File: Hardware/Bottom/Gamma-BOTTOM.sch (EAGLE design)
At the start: 33 parts

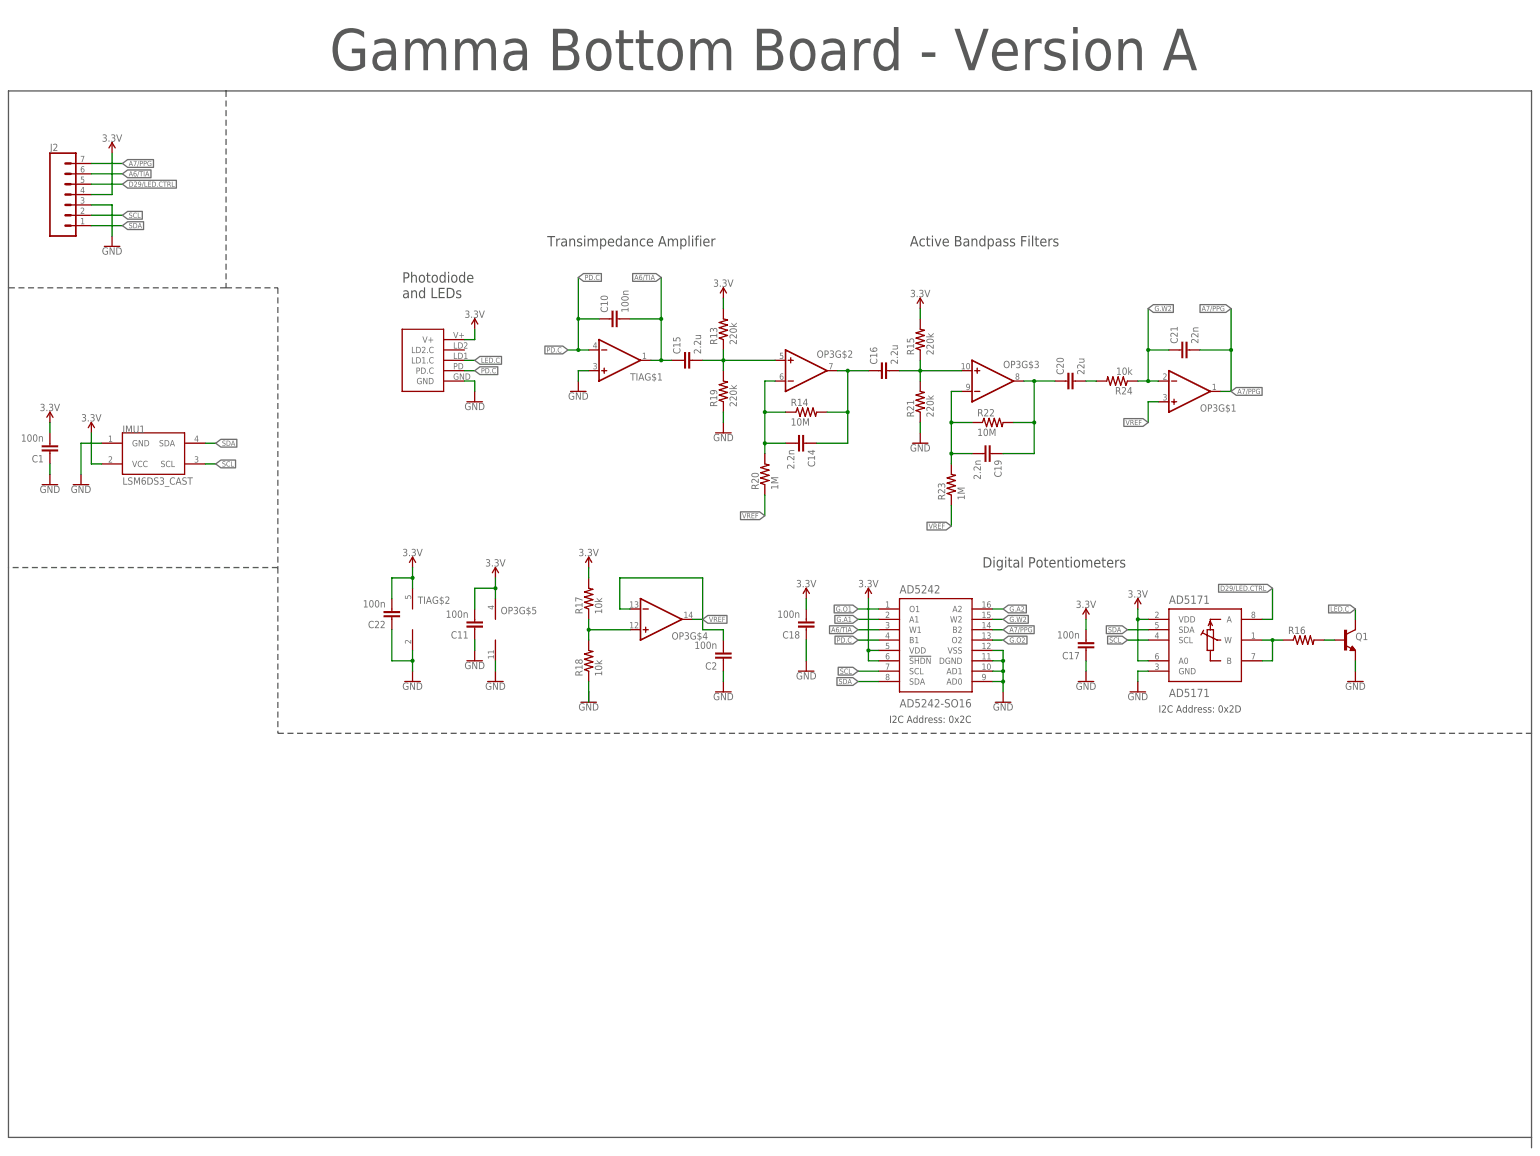
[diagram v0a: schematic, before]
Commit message: Pushed Changes to where I'm at (Take 007)
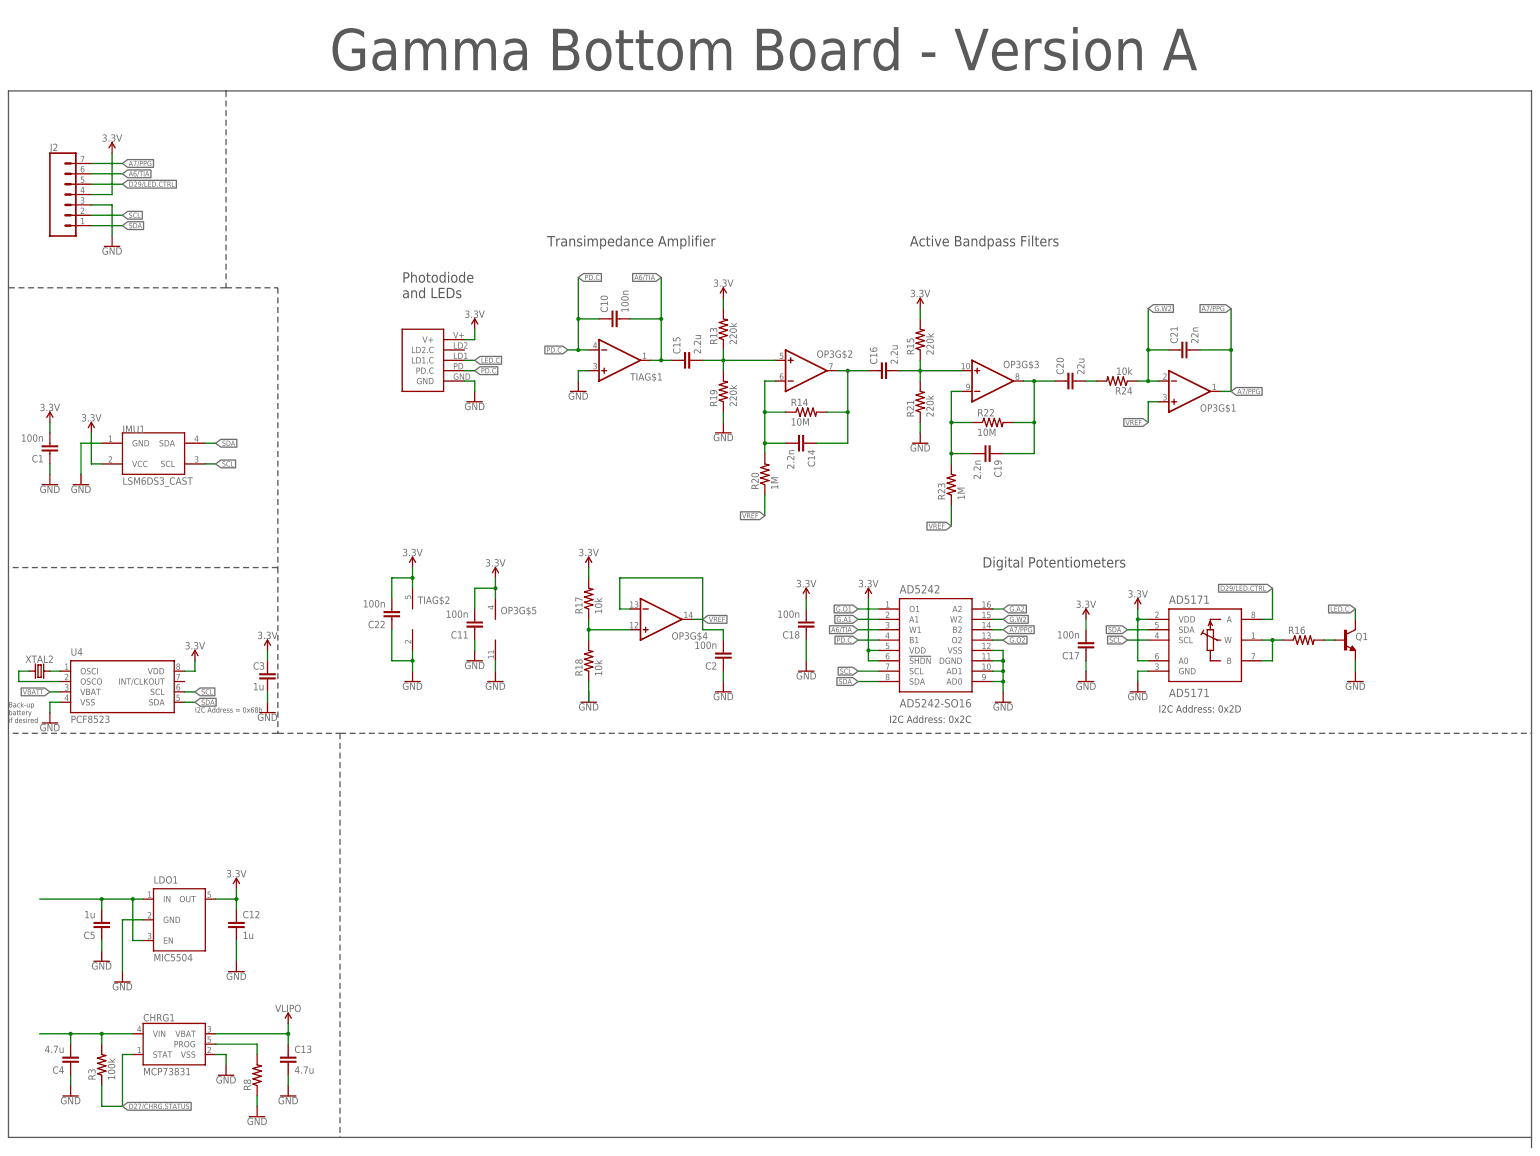
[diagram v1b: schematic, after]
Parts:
- added C12, C3, C5: 1u, LinnesLab-Passives:CAPACITOR0603
- added C13, C4: 4.7u, LinnesLab-Passives:CAPACITOR0603
- added CHRG1: MCP73831, LinnesLab-Power:MCP73831
- added LDO1: MIC5504, LinnesLab-Power:MIC5504
- added R3: 100k, LinnesLab-Passives:RESISTOR0603
- added R8: (no value), LinnesLab-Passives:RESISTOR0603
- added U4: PCF8523, LinnesLab-Clocks:PCF8523
- added XTAL2: 32.7680kHz, LinnesLab-Clocks:CRYSTALECS-.327-12.5-12-C-TR
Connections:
- new net D27/CHRG.STATUS: CHRG1.STAT, R3.1
- new net N$1: U4.OSCO, XTAL2.1
- new net N$2: U4.OSCI, XTAL2.2
- new net N$3: CHRG1.PROG, R8.2
- new net VBATT: U4.VBAT
- new net VIN1: C4.2, C5.2, CHRG1.VIN, LDO1.EN, LDO1.IN, R3.2
- new net VLIPO: C13.1, CHRG1.VBAT
- net 3.3V: now also C12.1, C3.1, LDO1.OUT, U4.VDD
- net GND: now also C12.2, C13.2, C3.2, C4.1, C5.1, CHRG1.VSS, LDO1.GND, R8.1, U4.VSS
- net SCL: now also U4.SCL
- net SDA: now also U4.SDA
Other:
- note added: "Back-up battery if desired"
- note added: "Bottom Board Power Management"
- note added: "I2C Address = 0x68h"
- note added: "Real-Time Clock"
